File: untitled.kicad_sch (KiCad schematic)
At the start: 19 parts, among them J4 motor

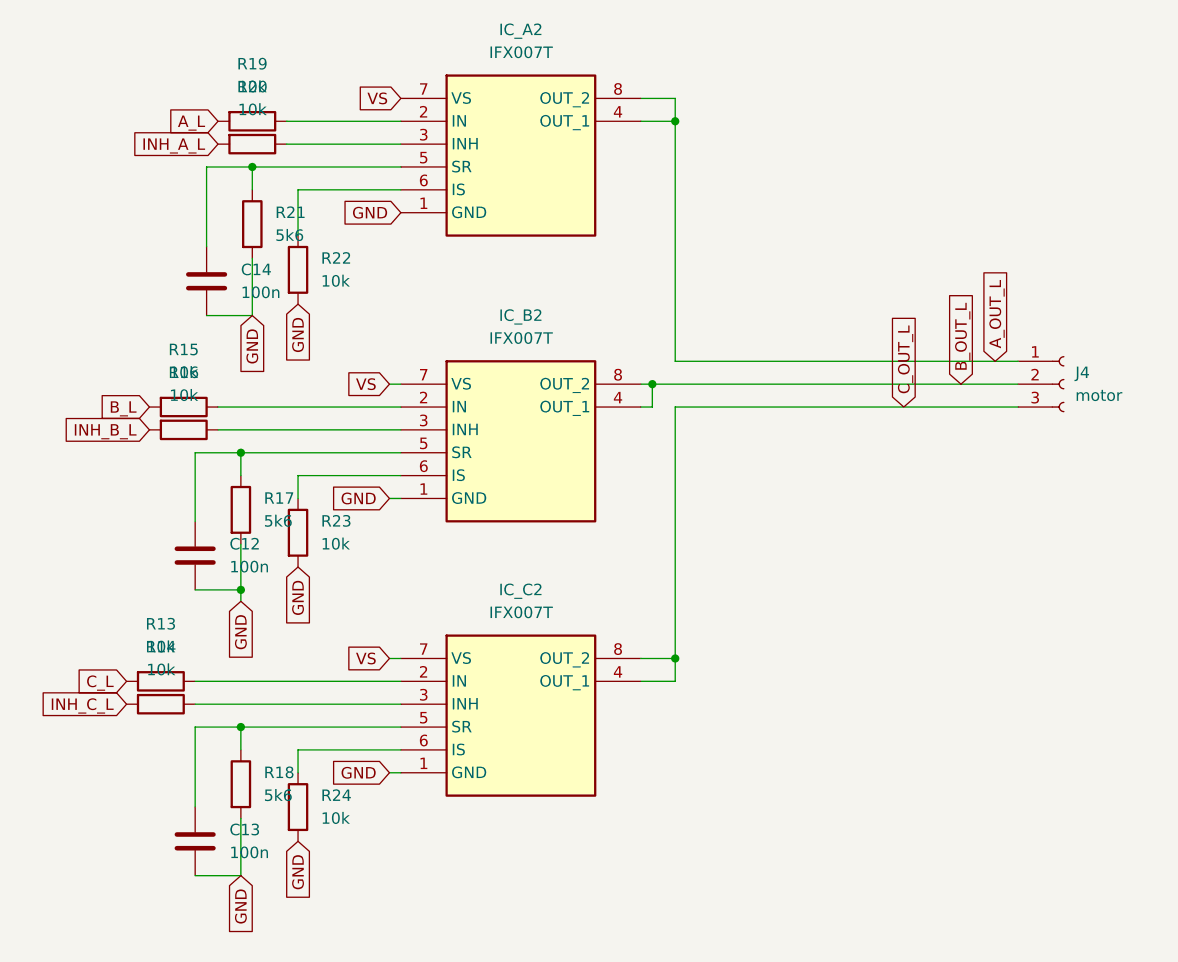
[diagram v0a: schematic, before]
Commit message: controller fw added, unfinished
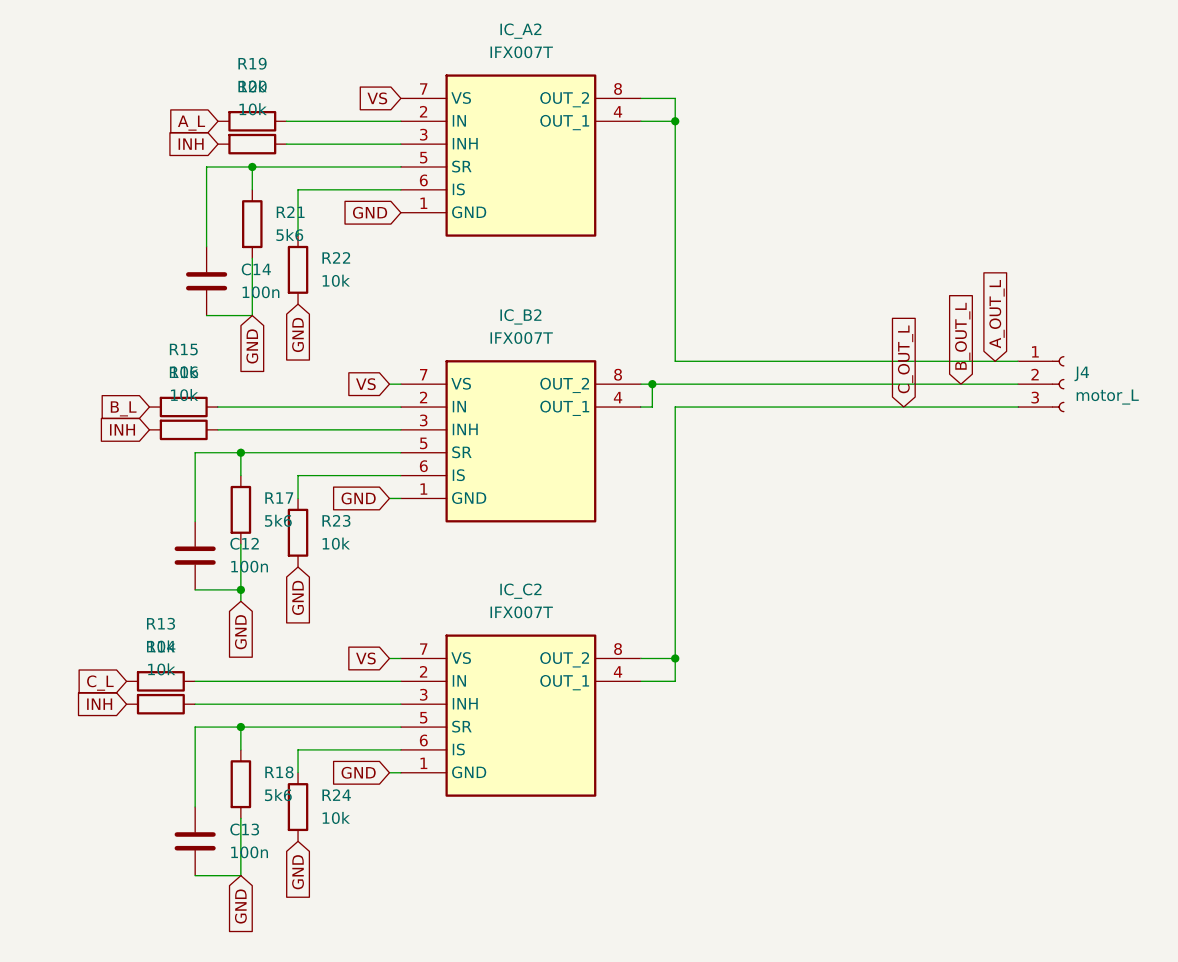
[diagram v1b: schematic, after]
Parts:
- J4: value motor -> motor_L
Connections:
- net INH_B_L is gone; now on net INH: R16.2
- net INH_C_L is gone; now on net INH: R14.2
- net INH_A_L renamed INH
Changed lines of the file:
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@@
 		)
 	)
-	(global_label "INH_C_L"
+	(global_label "INH"
 		(shape input)
 		(at 91.44 119.38 180)
@@
 		)
 		(property "Intersheetrefs" "${INTERSHEET_REFS}"
-			(at 80.9557 119.38 0)
+			(at 85.189 119.38 0)
 			(effects
 				(font
@@
 		)
 	)
-	(global_label "INH_A_L"
+	(global_label "INH"
 		(shape input)
 		(at 101.6 57.15 180)
@@
 		)
 		(property "Intersheetrefs" "${INTERSHEET_REFS}"
-			(at 91.2971 57.15 0)
+			(at 95.349 57.15 0)
 			(effects
 				(font
@@
 		)
 	)
-	(global_label "INH_B_L"
+	(global_label "INH"
 		(shape input)
 		(at 93.98 88.9 180)
@@
 		)
 		(property "Intersheetrefs" "${INTERSHEET_REFS}"
-			(at 83.4957 88.9 0)
+			(at 87.729 88.9 0)
 			(effects
 				(font
@@
 			)
 		)
-		(property "Value" "motor"
+		(property "Value" "motor_L"
 			(at 196.85 85.09 0)
 			(effects
